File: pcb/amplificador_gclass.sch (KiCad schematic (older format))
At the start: 49 parts, among them J1 Jack_3.5mm_5pin, P1 CONN_01X01, P10 CONN_01X01, P12 OUT, P13 CONN_01X01, P2 CONN_01X01, P3 CONN_01X01, P4 CONN_01X01, P5 +VA_GND, P6 +VB_GND, P7 -VA_GND, P8 -VB_GND, P9 CONN_01X01, Q1 MPSA56_PNP_EBC, Q10 MPSA06_NPN_EBC, Q11 MPSA56_PNP_EBC, Q12 MPSA06_NPN_EBC, Q2 MPSA56_PNP_EBC, Q3 MPSA06_NPN_EBC, Q4 MPSA56_PNP_EBC, Q5 MPSA06_NPN_EBC, Q6 MPSA56_PNP_EBC, Q7 MPSA56_PNP_EBC, Q8 MPSA56_PNP_EBC, Q9 MPSA56_PNP_EBC

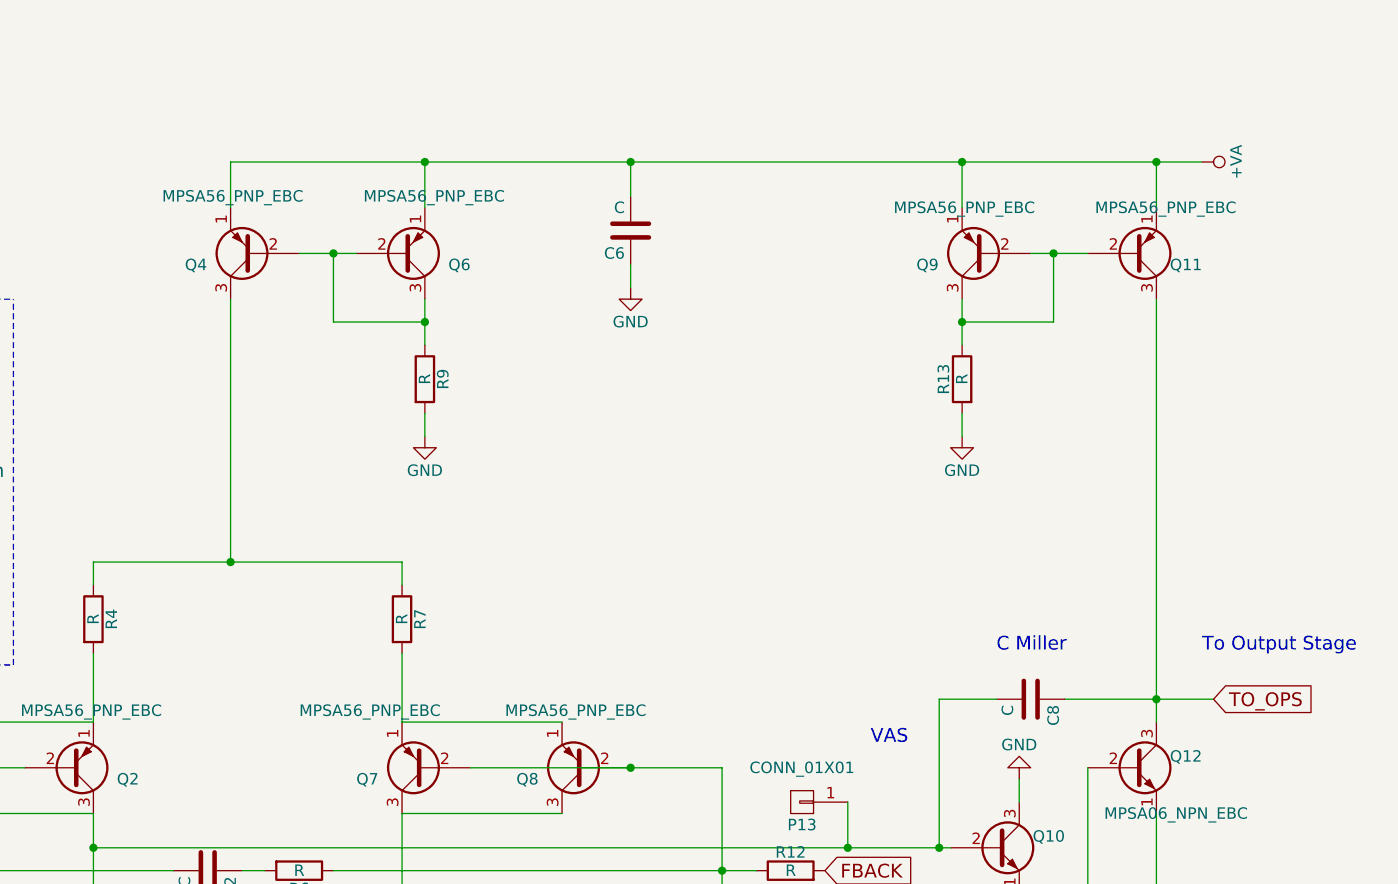
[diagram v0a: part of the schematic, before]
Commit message: Arreglando PCB
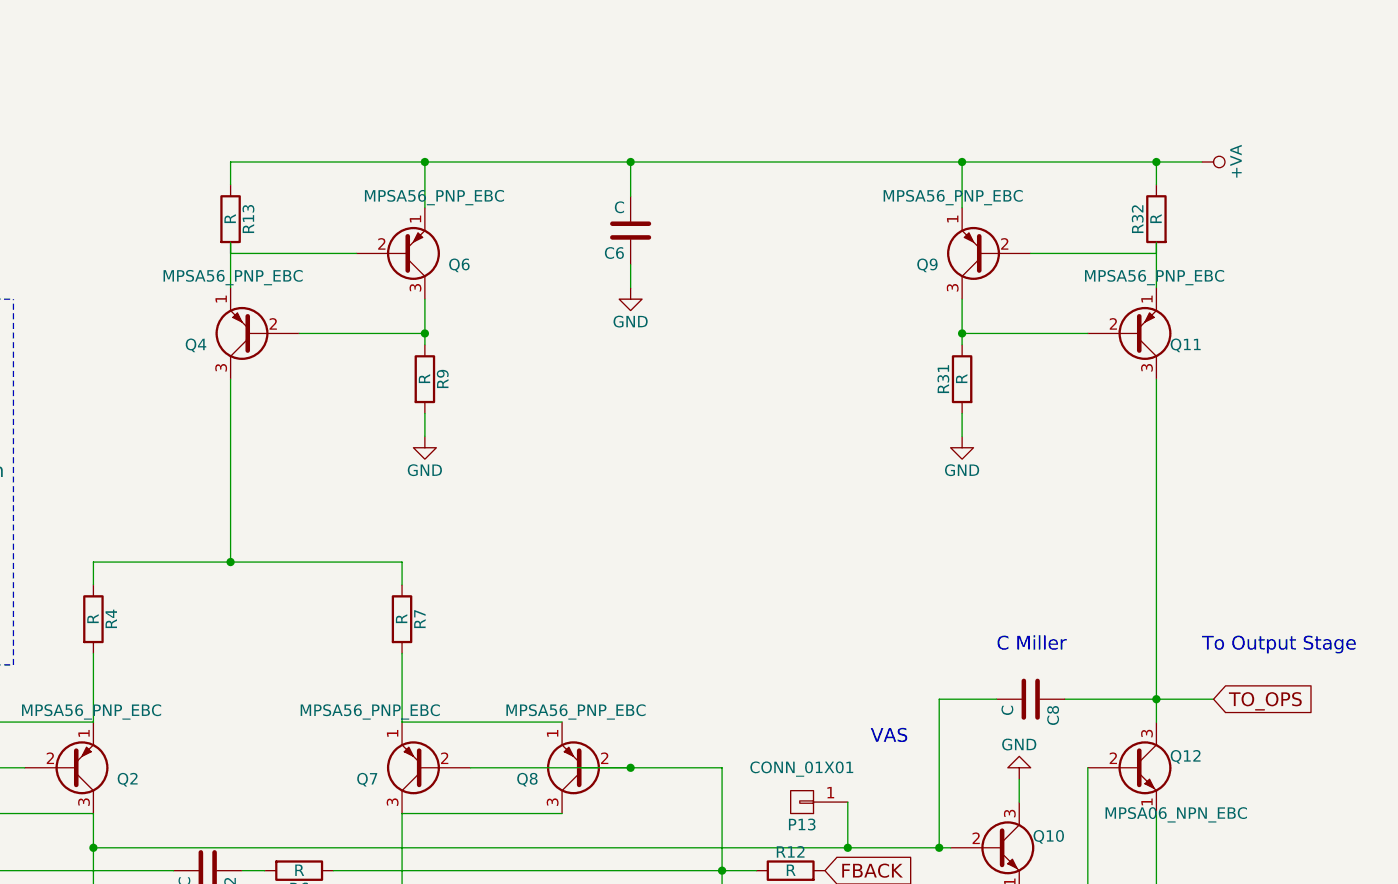
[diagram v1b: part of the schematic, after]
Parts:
- added R31, R32: R, Resistors_ThroughHole:Resistor_Horizontal_RM10mm, symbol R
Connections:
- net +VA: now also R13.1, R32.1; no longer Q11.1 (E), Q4.1 (E)
- net GND: now also R31.2; no longer R13.2
- net at Q4.2 (B), Q6.3 (C), R9.1: no longer Q6.2 (B)
- net at Q11.2 (B), Q9.3 (C): now also R31.1; no longer Q9.2 (B), R13.1
- new net: Q6.2 (B), R13.2
- new net: Q9.2 (B), R32.2
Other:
- moved on the sheet: Q4
